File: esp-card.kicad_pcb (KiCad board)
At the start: 2 copper layers, 85 x 55 mm, 54 parts, among them J2 Conn_01x04_Socket, U1 NH-B1010RGBT-HF, U2 ESP32-C3FH4, U3 NH-B1010RGBT-HF, U4 TS-1187A-B-A-B, U5 TS-1187A-B-A-B, U58 TS-1187A-B-A-B, U59 YTC-TC16-30, U60 AMS1117-3_3, U61 NH-B1010RGBT-HF, U62 NH-B1010RGBT-HF, U63 NH-B1010RGBT-HF, U64 NH-B1010RGBT-HF, U65 NH-B1010RGBT-HF, U66 NH-B1010RGBT-HF, U67 NH-B1010RGBT-HF, U68 NH-B1010RGBT-HF, U69 NH-B1010RGBT-HF, U70 NH-B1010RGBT-HF, U71 NH-B1010RGBT-HF, U72 NH-B1010RGBT-HF, U73 TS-1187A-B-A-B, X1 CF4040M00015001

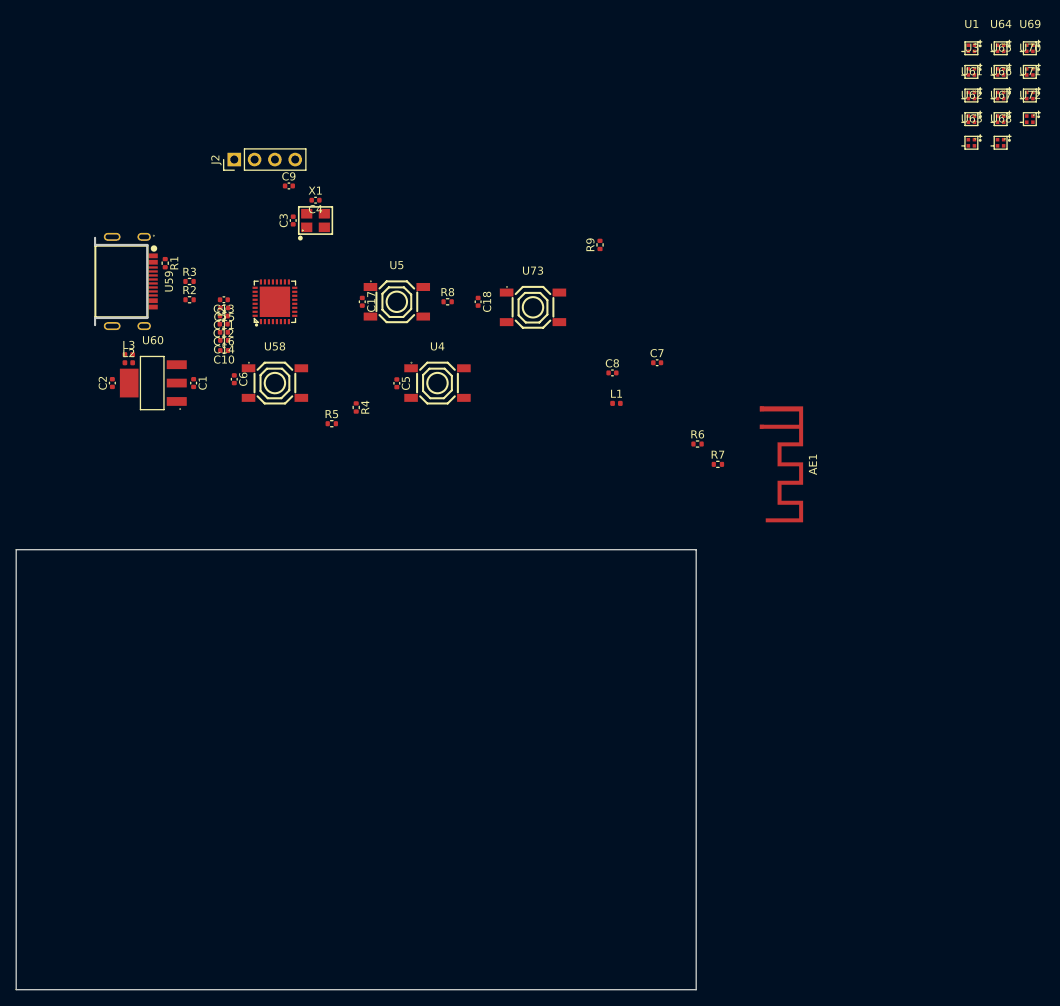
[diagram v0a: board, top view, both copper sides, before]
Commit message: better routing
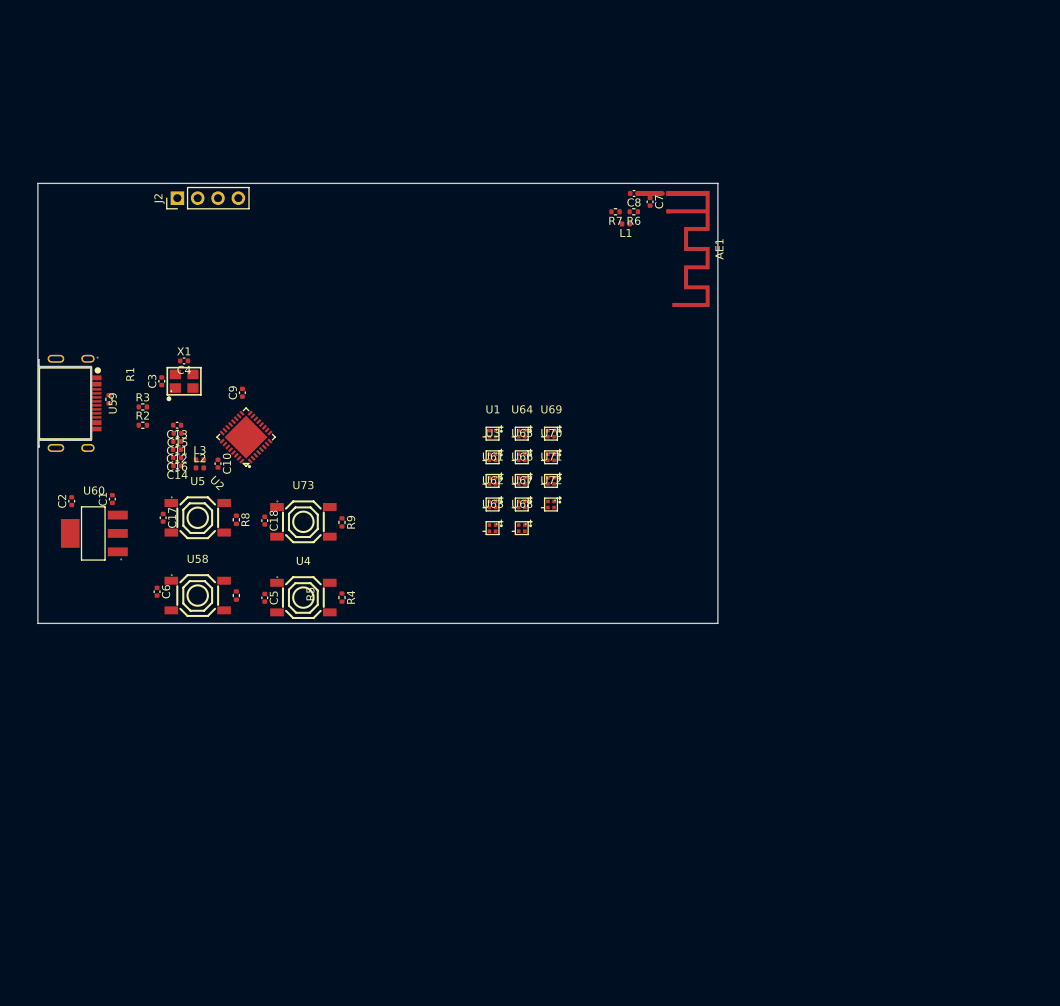
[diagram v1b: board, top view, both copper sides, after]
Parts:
- L1: value 2nH -> 2.2nH
- moved U1 76.8 mm to (166.9, 105.4)
- moved U3 76.8 mm to (166.9, 108.3)
- moved U64 76.8 mm to (170.6, 105.4)
- moved U65 76.8 mm to (170.6, 108.3)
- moved U69 76.8 mm to (174.2, 105.4)
- moved U70 76.8 mm to (174.2, 108.3)
- moved U61 76.8 mm to (166.9, 111.3)
- moved U62 76.8 mm to (166.9, 114.2)
- moved U63 76.8 mm to (166.9, 117.2)
- moved U66 76.8 mm to (170.6, 111.3)
- moved U67 76.8 mm to (170.6, 114.2)
- moved U68 76.8 mm to (170.6, 117.2)
- moved U71 76.8 mm to (174.2, 111.3)
- moved U72 76.8 mm to (174.2, 114.2)
- moved R9 47.4 mm to (148.1, 116.5), turned to -90 degrees
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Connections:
- C10 pad 1: Net-(D2-A) -> Net-(C10-Pad1)
- L2 pad 2: Net-(D2-A) -> Net-(C10-Pad1)
- L3 pad 2: Net-(D2-A) -> Net-(C10-Pad1)
- U2 pad 2: Net-(D2-K) -> Net-(C10-Pad1)
- U2 pad 3: Net-(D2-K) -> Net-(C10-Pad1)
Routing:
- net GND: track 0.00 -> 3.05 mm
